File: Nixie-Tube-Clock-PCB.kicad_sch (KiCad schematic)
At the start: 71 parts, among them J1 Conn_01x11_Socket, J2 Conn_01x11_Socket, J3 Conn_01x11_Socket, J4 Conn_01x11_Socket, J5 Conn_01x11_Socket, J6 Conn_01x11_Socket, J7 Barrel_Jack_MountingPin, U1 74HC595, U10 74HC595, U3 74HC595, U4 LMR33630BDDAR, U5 DS1307N+

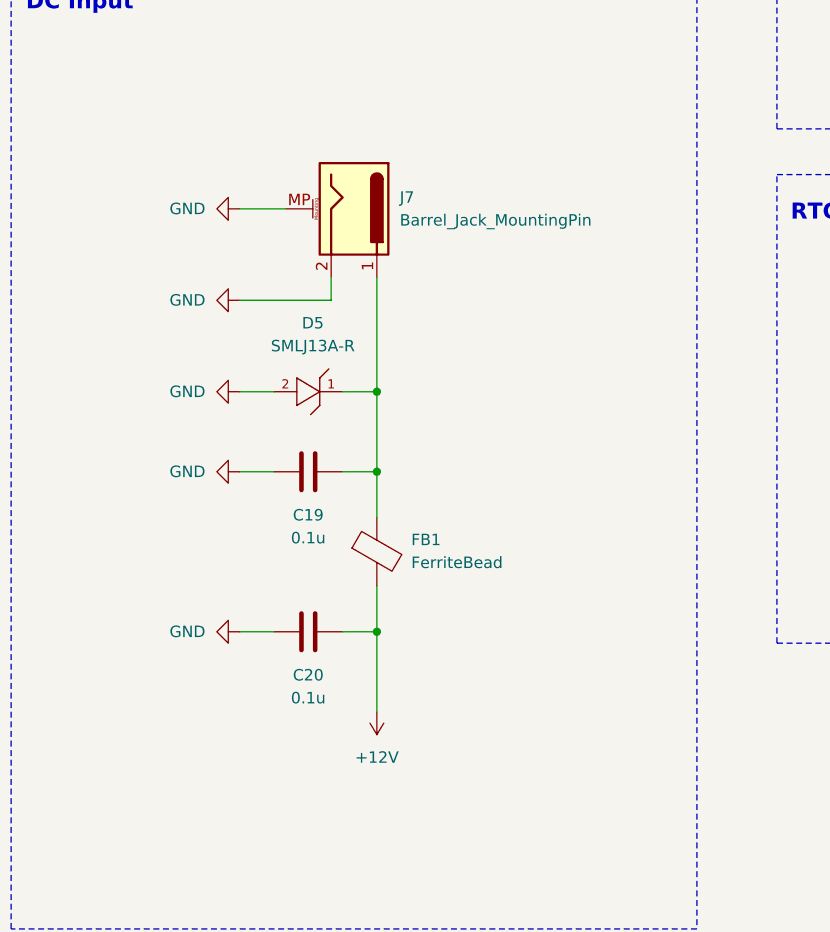
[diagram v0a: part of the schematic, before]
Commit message: edit
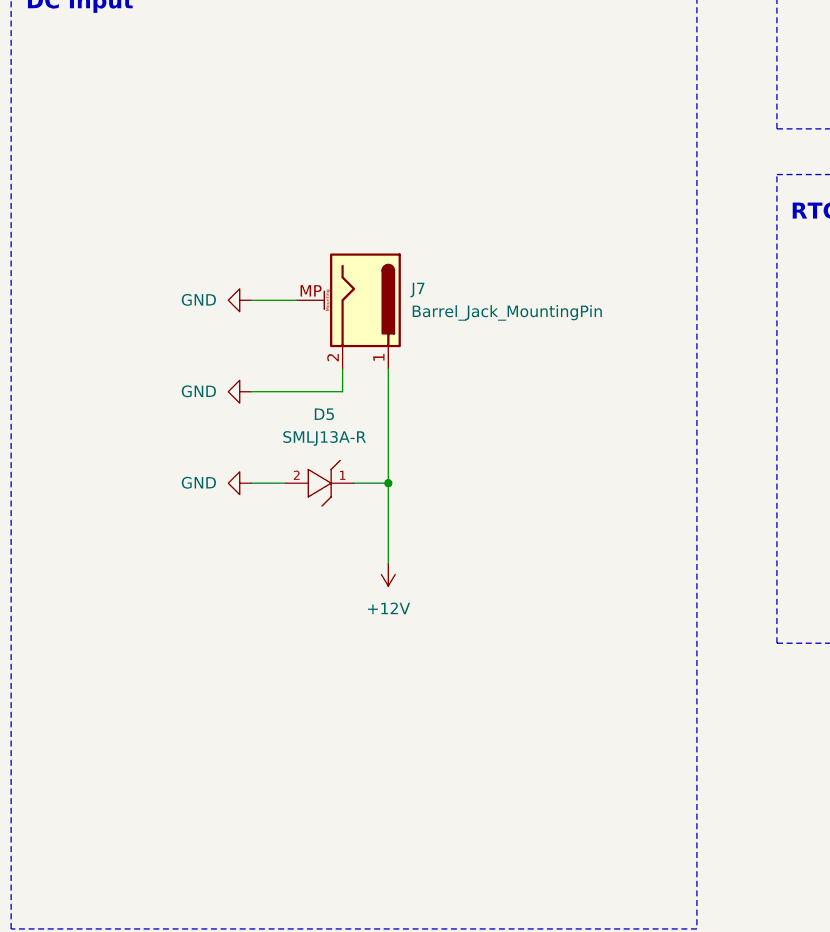
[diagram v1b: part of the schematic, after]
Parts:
- removed C19, C20: 0.1u, Capacitor_SMD:C_0402_1005Metric_Pad0.74x0.62mm_HandSolder, symbol Device:C
- removed FB1: FerriteBead, symbol Device:FerriteBead
- C10, C11: footprint (none) -> Capacitor_THT:C_Rect_L33.0mm_W20.0mm_P27.50mm_MKS4
- C12, C21, C6: footprint (none) -> Capacitor_SMD:C_0402_1005Metric_Pad0.74x0.62mm_HandSolder
- C22, C23, C5, C8: footprint (none) -> Capacitor_SMD:C_0603_1608Metric_Pad1.08x0.95mm_HandSolder
- C24, C25, C4: footprint (none) -> Capacitor_SMD:C_1210_3225Metric_Pad1.33x2.70mm_HandSolder
- C7: footprint (none) -> Capacitor_SMD:C_1206_3216Metric_Pad1.33x1.80mm_HandSolder
- C9: footprint (none) -> Capacitor_SMD:C_1206_3216Metric
- L1, L2: footprint (none) -> Inductor_SMD:L_Bourns_SRR1260
- R10: footprint (none) -> Resistor_SMD:R_0805_2012Metric_Pad1.20x1.40mm_HandSolder
- R11, R12, R13, R14, R15: footprint (none) -> Resistor_SMD:R_0815_2038Metric_Pad1.20x4.05mm_HandSolder
- R16, R8: footprint (none) -> Resistor_SMD:R_1206_3216Metric_Pad1.30x1.75mm_HandSolder
- R17, R4, R5, R6, R7, R9: footprint (none) -> Resistor_SMD:R_0603_1608Metric_Pad0.98x0.95mm_HandSolder
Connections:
- net +12V: now also D5.1, J7.1
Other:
- moved on the sheet: D5, J7
